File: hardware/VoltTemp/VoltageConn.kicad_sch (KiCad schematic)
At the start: 25 parts, among them J11 Conn_01x07

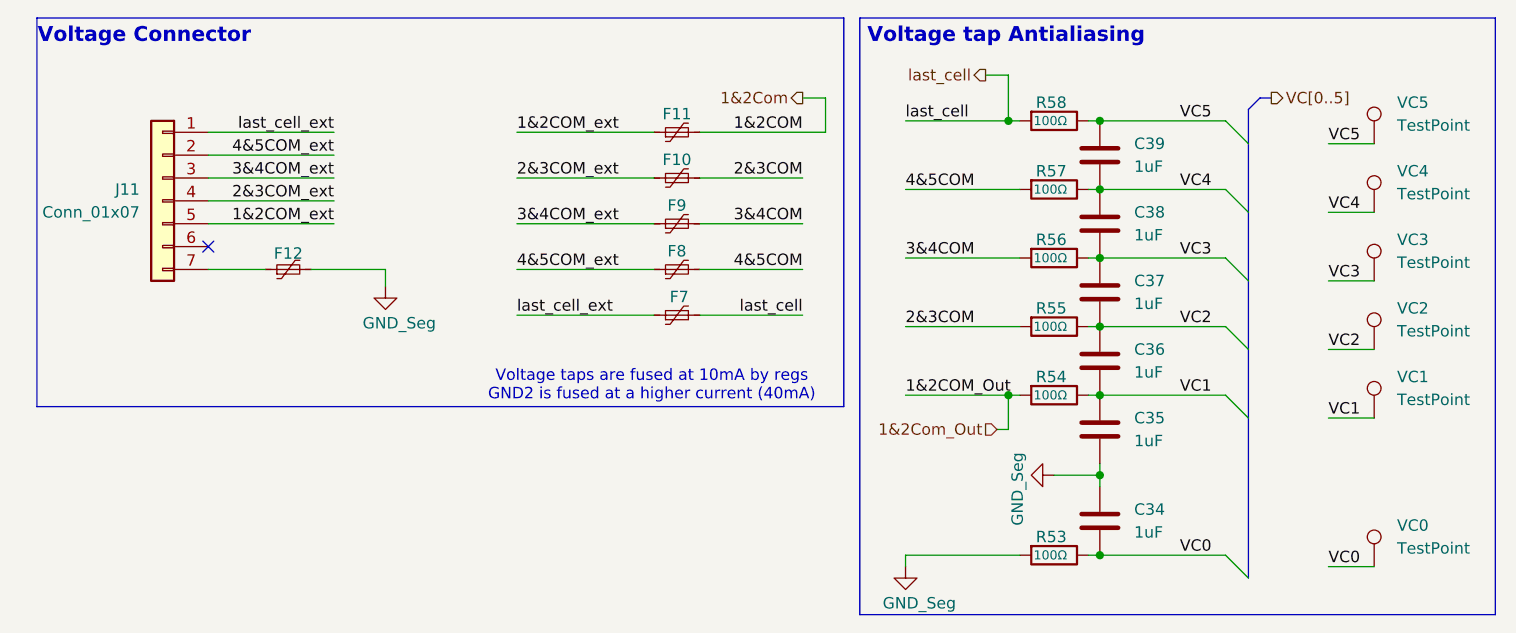
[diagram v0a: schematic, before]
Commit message: jlcpcb assembly files
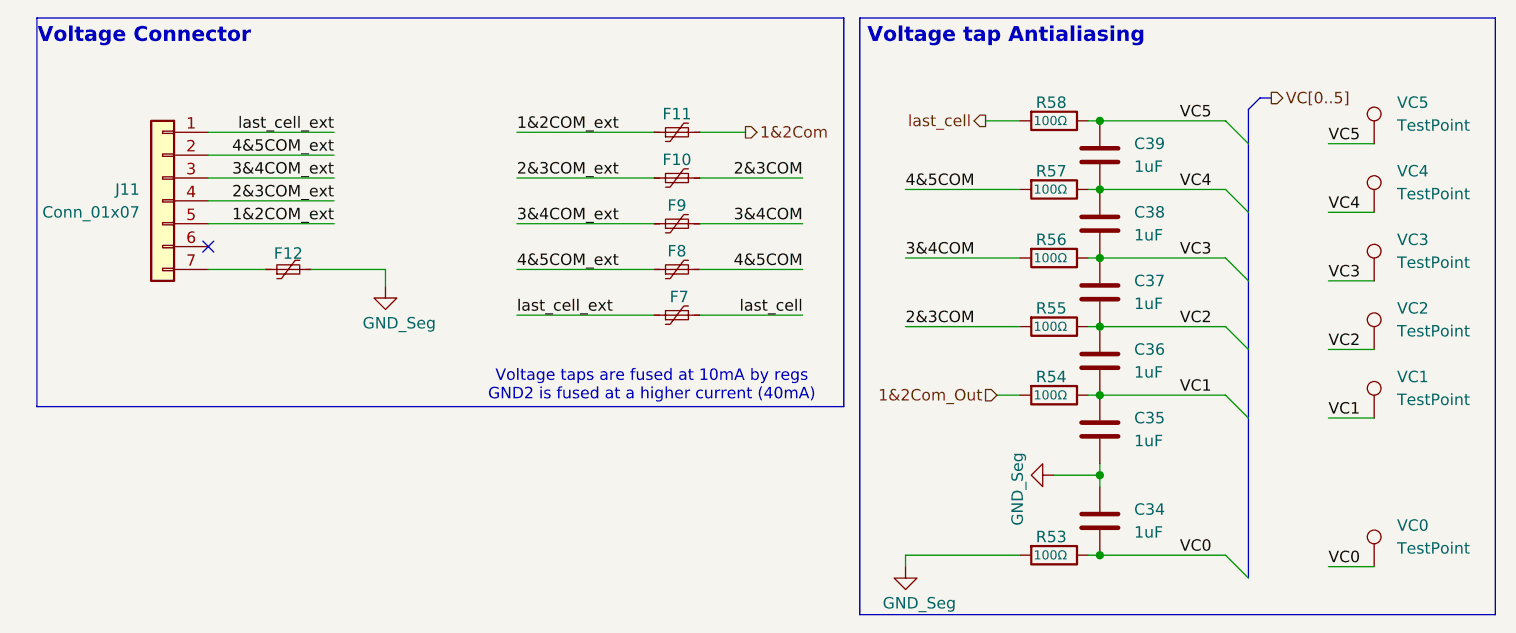
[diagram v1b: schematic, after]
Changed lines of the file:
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@@
-	)
-	(junction
-		(at 125.73 74.93)
-		(diameter 0)
-		(color 0 0 0 0)
 	)
 	(junction
@@
 	)
 	(junction
-		(at 125.73 44.45)
-		(diameter 0)
-		(color 0 0 0 0)
-	)
-	(junction
 		(at 135.89 74.93)
 		(diameter 0)
@@
 		)
 	)
-	(wire
-		(pts
-			(xy 105.41 41.91) (xy 105.41 45.72)
-		)
-		(stroke
-			(width 0)
-			(type default)
-		)
-	)
 	(bus
 		(pts
@@
 		)
 	)
+	(wire
+		(pts
+			(xy 91.44 45.72) (xy 96.52 45.72)
+		)
+		(stroke
+			(width 0)
+			(type default)
+		)
+	)
 	(bus
 		(pts
@@
 	(wire
 		(pts
-			(xy 125.73 74.93) (xy 127 74.93)
-		)
-		(stroke
-			(width 0)
-			(type default)
-		)
-	)
-	(wire
-		(pts
 			(xy 114.3 52.07) (xy 127 52.07)
 		)
@@
 	(wire
 		(pts
-			(xy 125.73 39.37) (xy 125.73 44.45)
-		)
-		(stroke
-			(width 0)
-			(type default)
-		)
-	)
-	(wire
-		(pts
 			(xy 71.12 45.72) (xy 86.36 45.72)
 		)
@@
 		)
 	)
-	(wire
-		(pts
-			(xy 91.44 45.72) (xy 105.41 45.72)
-		)
-		(stroke
-			(width 0)
-			(type default)
-		)
-	)
 	(bus
 		(pts
@@
 	(wire
 		(pts
-			(xy 114.3 44.45) (xy 125.73 44.45)
-		)
-		(stroke
-			(width 0)
-			(type default)
-		)
-	)
-	(wire
-		(pts
 			(xy 134.62 74.93) (xy 135.89 74.93)
 		)
@@
 	(wire
 		(pts
-			(xy 102.87 41.91) (xy 105.41 41.91)
-		)
-		(stroke
-			(width 0)
-			(type default)
-		)
-	)
-	(wire
-		(pts
 			(xy 161.29 54.61) (xy 166.37 54.61)
 		)
@@
 	(wire
 		(pts
-			(xy 124.46 78.74) (xy 125.73 78.74)
-		)
-		(stroke
-			(width 0)
-			(type default)
-		)
-	)
-	(wire
-		(pts
-			(xy 125.73 44.45) (xy 127 44.45)
+			(xy 124.46 74.93) (xy 127 74.93)
 		)
 		(stroke
@@
 	(wire
 		(pts
-			(xy 125.73 74.93) (xy 125.73 78.74)
-		)
-		(stroke
-			(width 0)
-			(type default)
-		)
-	)
-	(wire
-		(pts
 			(xy 135.89 83.82) (xy 135.89 85.09)
 		)
@@
 	(wire
 		(pts
-			(xy 123.19 39.37) (xy 125.73 39.37)
+			(xy 123.19 44.45) (xy 127 44.45)
 		)
 		(stroke
@@
 	(wire
 		(pts
-			(xy 114.3 74.93) (xy 125.73 74.93)
-		)
-		(stroke
-			(width 0)
-			(type default)
-		)
-	)
-	(wire
-		(pts
 			(xy 71.12 55.88) (xy 86.36 55.88)
 		)
@@
 			(width 0)
 			(type default)
-		)
-	)
-	(label "1&2COM_Out"
-		(at 114.3 74.93 0)
-		(effects
-			(font
-				(size 1.27 1.27)
-			)
-			(justify left bottom)
 		)
 	)
@@
 		)
 	)
-	(label "last_cell"
-		(at 114.3 44.45 0)
-		(effects
-			(font
-				(size 1.27 1.27)
-			)
-			(justify left bottom)
-		)
-	)
 	(label "VC2"
 		(at 144.78 67.31 0)
@@
 	(label "2&3COM"
 		(at 102.87 50.8 180)
-		(effects
-			(font
-				(size 1.27 1.27)
-			)
-			(justify right bottom)
-		)
-	)
-	(label "1&2COM"
-		(at 102.87 45.72 180)
 		(effects
 			(font
@@
 	(hierarchical_label "last_cell"
 		(shape output)
-		(at 123.19 39.37 180)
+		(at 123.19 44.45 180)
 		(effects
 			(font
@@
 	(hierarchical_label "1&2Com"
 		(shape output)
-		(at 102.87 41.91 180)
-		(effects
-			(font
-				(size 1.27 1.27)
-			)
-			(justify right)
+		(at 96.52 45.72 0)
+		(effects
+			(font
+				(size 1.27 1.27)
+			)
+			(justify left)
 		)
 	)
 	(hierarchical_label "1&2Com_Out"
 		(shape input)
-		(at 124.46 78.74 180)
-		(effects
-			(font
+		(at 124.46 74.93 180)
+		(effects
+			(font
